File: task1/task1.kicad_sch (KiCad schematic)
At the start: 13 parts, among them SW1 SW_Push, SW2 SW_Push, SW3 SW_Push

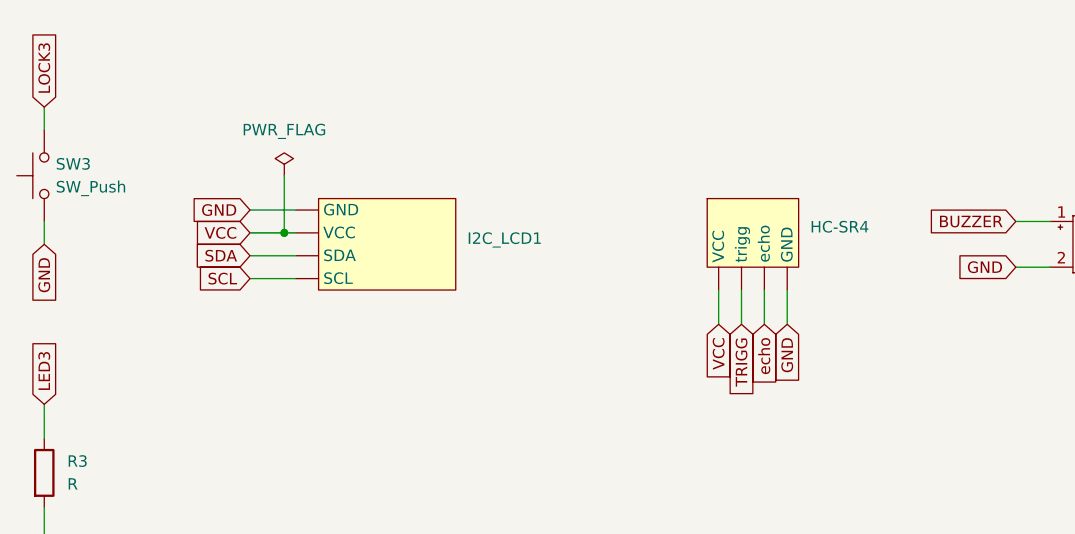
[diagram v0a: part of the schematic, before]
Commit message: cc
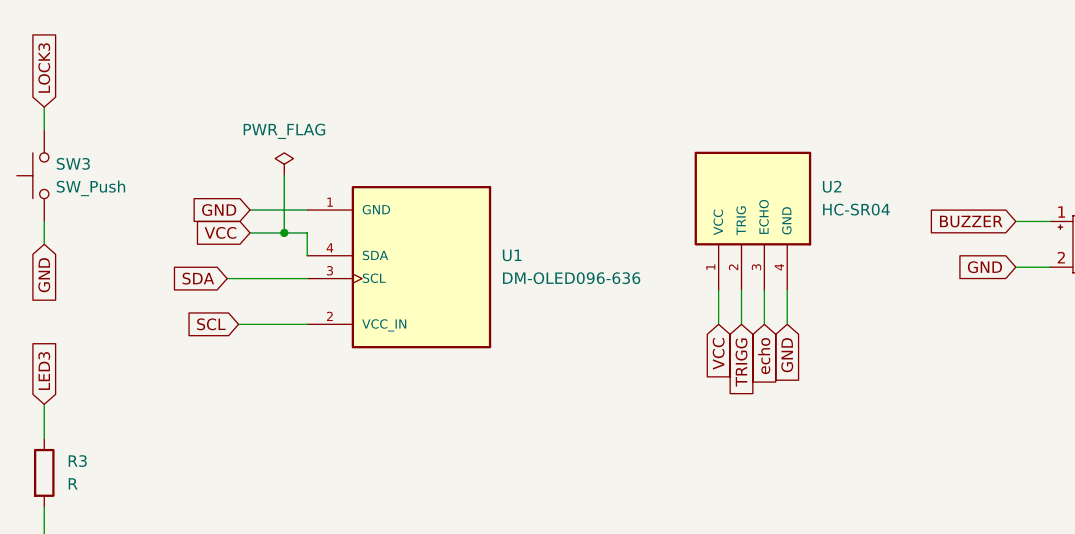
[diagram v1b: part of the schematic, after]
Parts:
- removed HC-SR4: ~, footprint and symbols:XCVR_HC-SR04, symbol sensors:HC-SR04
- removed I2C_LCD1: ~, footprint and symbols:LCD9-1.5-30X19.5MM, symbol LCD:I2C_LCD
- added U1: DM-OLED096-636, Display:I2C_LCD(OLED), symbol DM-OLED096-636:DM-OLED096-636
- added U2: HC-SR04, Sensor:HC-SR04, symbol HC-SR04:HC-SR04
- D1, D2, D3: footprint LED_SMD:LED_0201_0603Metric_Pad0.64x0.40mm_HandSolder -> LED_THT:LED_D1.8mm_W1.8mm_H2.4mm_Horizontal_O1.27mm_Z1.6mm
- R1, R2, R3: footprint Resistor_THT:R_Axial_DIN0204_L3.6mm_D1.6mm_P1.90mm_Vertical -> Resistor_THT:R_Axial_DIN0207_L6.3mm_D2.5mm_P7.62mm_Horizontal
- SW1, SW2, SW3: footprint footprint and symbols:SW_1825910-6-4 -> Button_Switch_THT:SW_PUSH_6mm_H8mm
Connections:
- net GND: now also U1.1 (GND), U2.4 (GND)
- net SCL: now also U1.2 (VCC_IN)
- net SDA: now also U1.3 (SCL)
- net TRIGG: now also U2.2 (TRIG)
- net VCC: now also U1.4 (SDA), U2.1 (VCC)
- net echo: now also U2.3 (ECHO)
